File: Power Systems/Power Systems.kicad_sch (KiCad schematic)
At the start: 16 parts, among them J1 CURRENT SENSE, J1 MOTOR DRIVER 1, J2 MOTOR DRIVER 2, J3 MOTOR DRIVER 3, J4 MOTOR DRIVER 4, K1 E-STOP RELAY 30A, SW1 MAIN DISCONECT - 30A, SW2 E-STOP NC

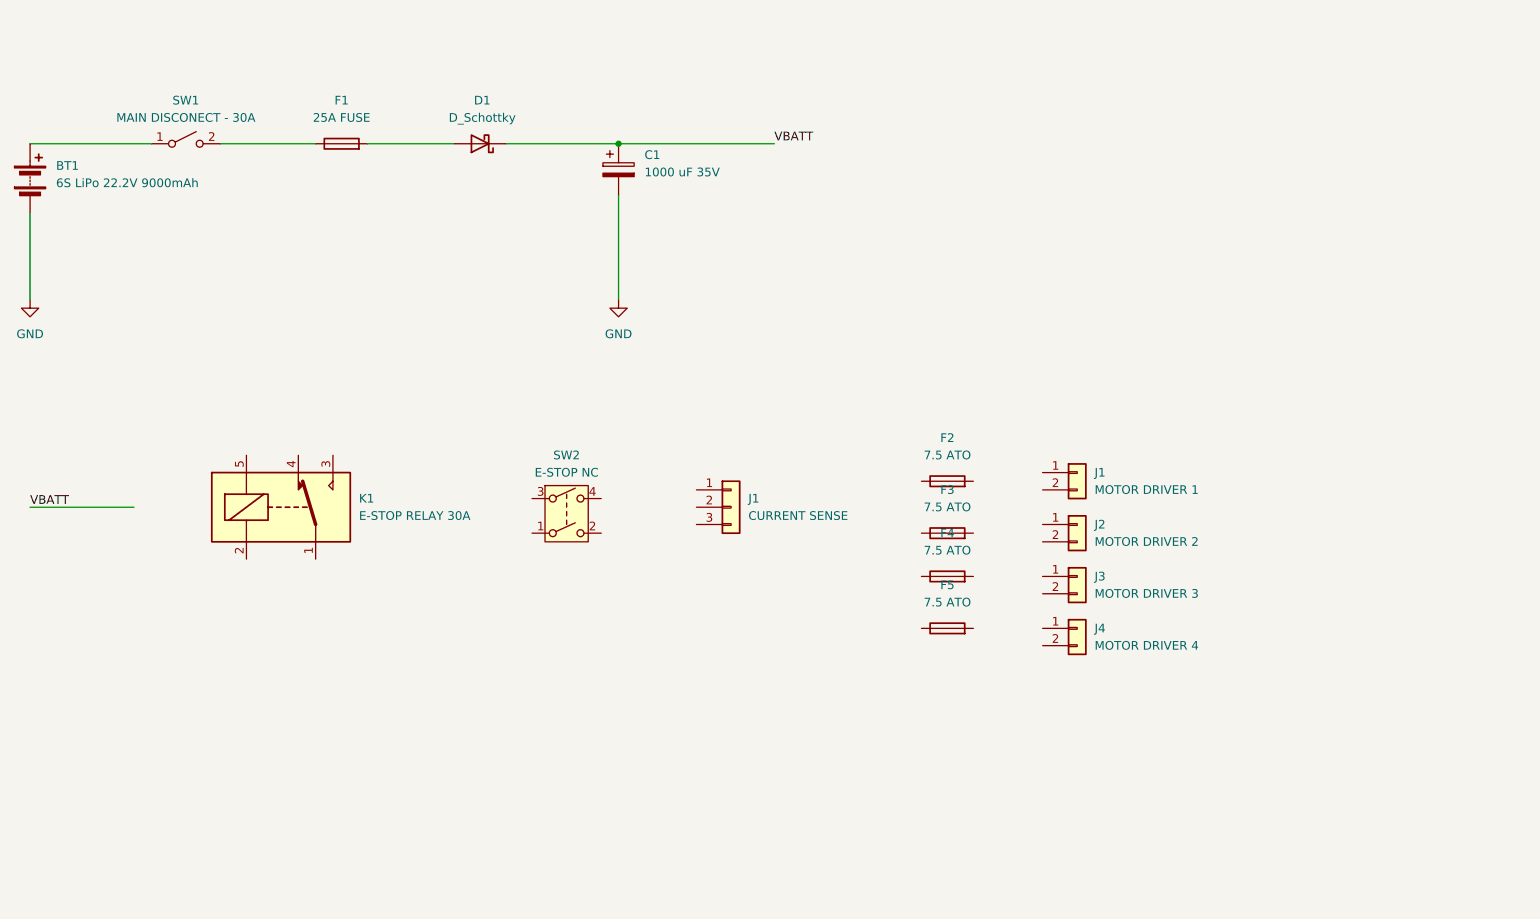
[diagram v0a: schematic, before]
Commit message: Motor driver
---
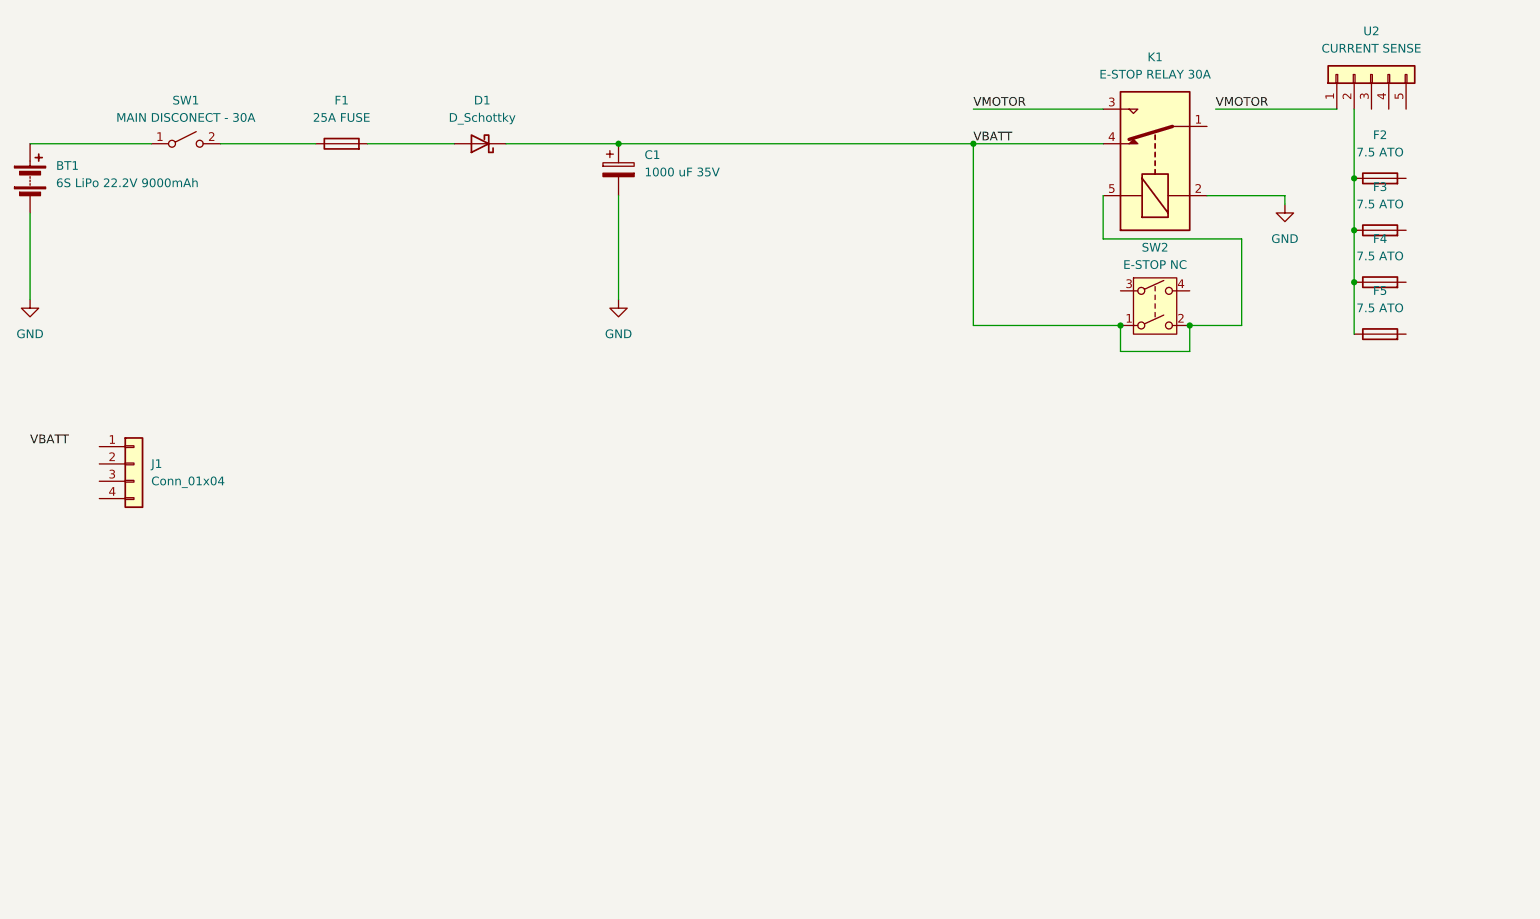
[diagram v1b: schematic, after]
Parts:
- removed J1: CURRENT SENSE, symbol Connector_Generic:Conn_01x03
- removed J1: MOTOR DRIVER 1, symbol Connector_Generic:Conn_01x02
- removed J2: MOTOR DRIVER 2, symbol Connector_Generic:Conn_01x02
- removed J3: MOTOR DRIVER 3, symbol Connector_Generic:Conn_01x02
- removed J4: MOTOR DRIVER 4, symbol Connector_Generic:Conn_01x02
- added J1: Conn_01x04, Package_TO_SOT_THT:TO-220-15_P2.54x5.08mm_StaggerOdd_Lead4.58mm_Vertical, symbol Connector_Generic:Conn_01x04
- added U2: CURRENT SENSE, symbol Connector_Generic:Conn_01x05
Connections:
- net GND: now also K1.2
- net VBATT: now also K1.4, K1.5, SW2.1, SW2.2
- net at F4.1: now also F2.1, F3.1, F5.1, U2.2 (Pin_2)
- net VMOTOR: now reaches K1.3
- net VMOTOR: now also U2.1 (Pin_1)
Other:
- moved on the sheet: F2, F3, F4, F5, K1, SW2

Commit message: f
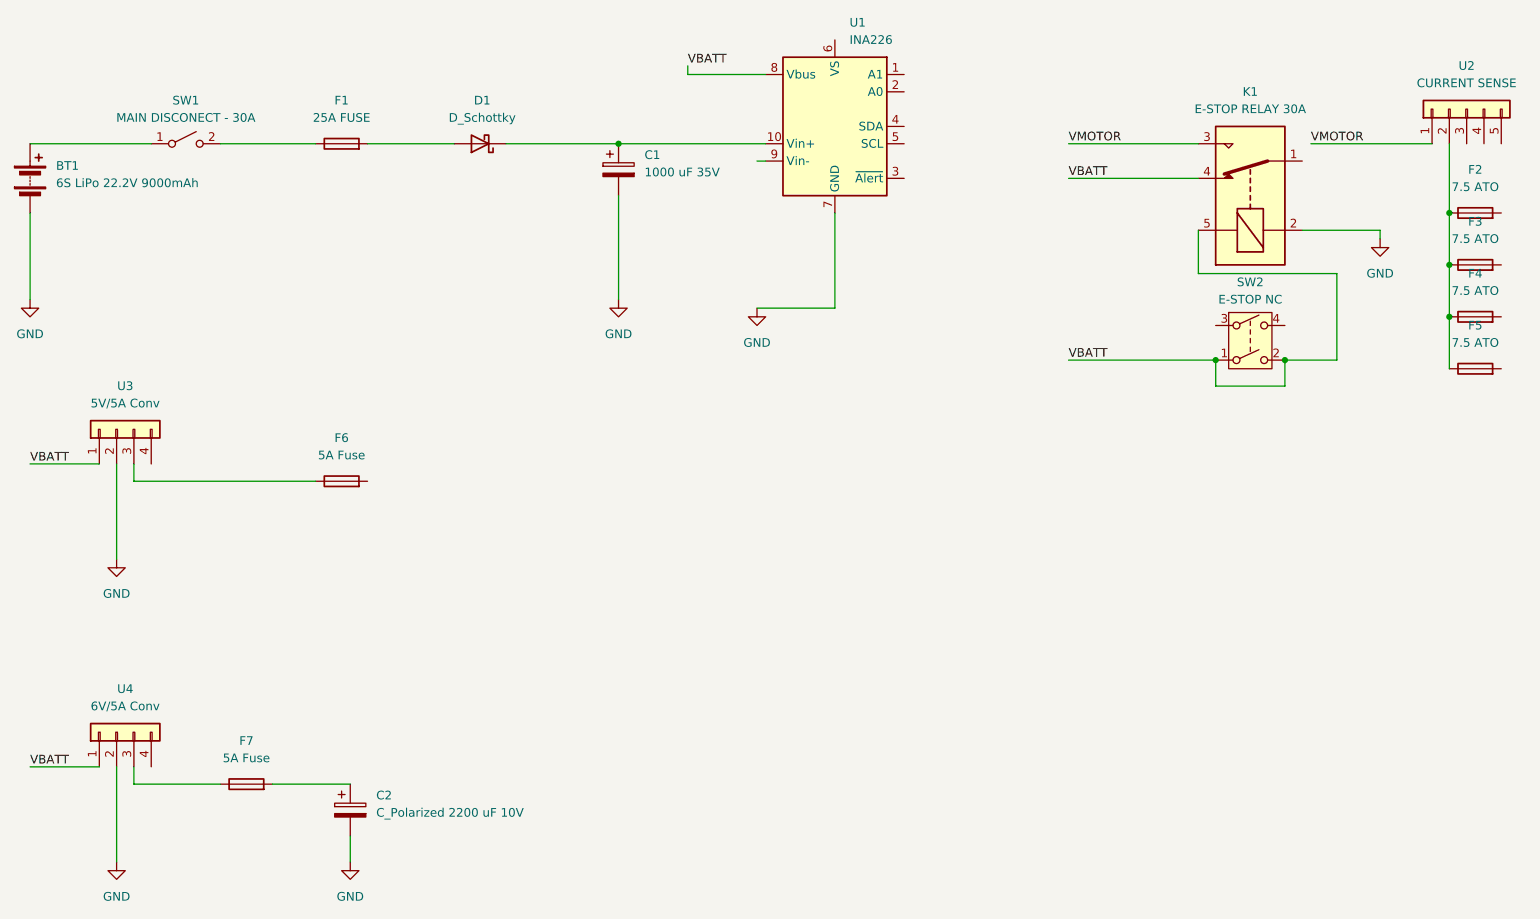
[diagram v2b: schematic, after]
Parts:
- added C2: C_Polarized 2200 uF 10V, symbol Device:C_Polarized
- added F6, F7: 5A Fuse, Package_LCC:PLCC-84_29.3x29.3mm_P1.27mm, symbol Device:Fuse
- added U1: INA226, Package_SO:TSSOP-10_3x3mm_P0.5mm, symbol Sensor_Energy:INA226
- added U4: 6V/5A Conv, Package_TO_SOT_THT:TO-220-15_P2.54x5.08mm_StaggerOdd_Lead4.58mm_Vertical, symbol Connector_Generic:Conn_01x04
- U3: renamed from J1; value Conn_01x04 -> 5V/5A Conv
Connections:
- net GND: now also U3.2 (Pin_2), C2.2, U1.7 (GND), U4.2 (Pin_2)
- net VBATT: now also U3.1 (Pin_1), U1.8 (Vbus), U4.1 (Pin_1); no longer C1.1, D1.1 (K)
- net at U3.3 (Pin_3): now also F6.1
- new net: C1.1, D1.1 (K), U1.10 (Vin+)
- new net: F7.1, U4.3 (Pin_3)
- new net: C2.1, F7.2
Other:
- moved on the sheet: F2, F3, F4, F5, K1, SW2, U2, U3
